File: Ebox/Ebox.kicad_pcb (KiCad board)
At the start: 2 copper layers, 61 x 53.3 mm, 3 parts, among them J1 Screw_Terminal_01x12, J2 Screw_Terminal_01x12

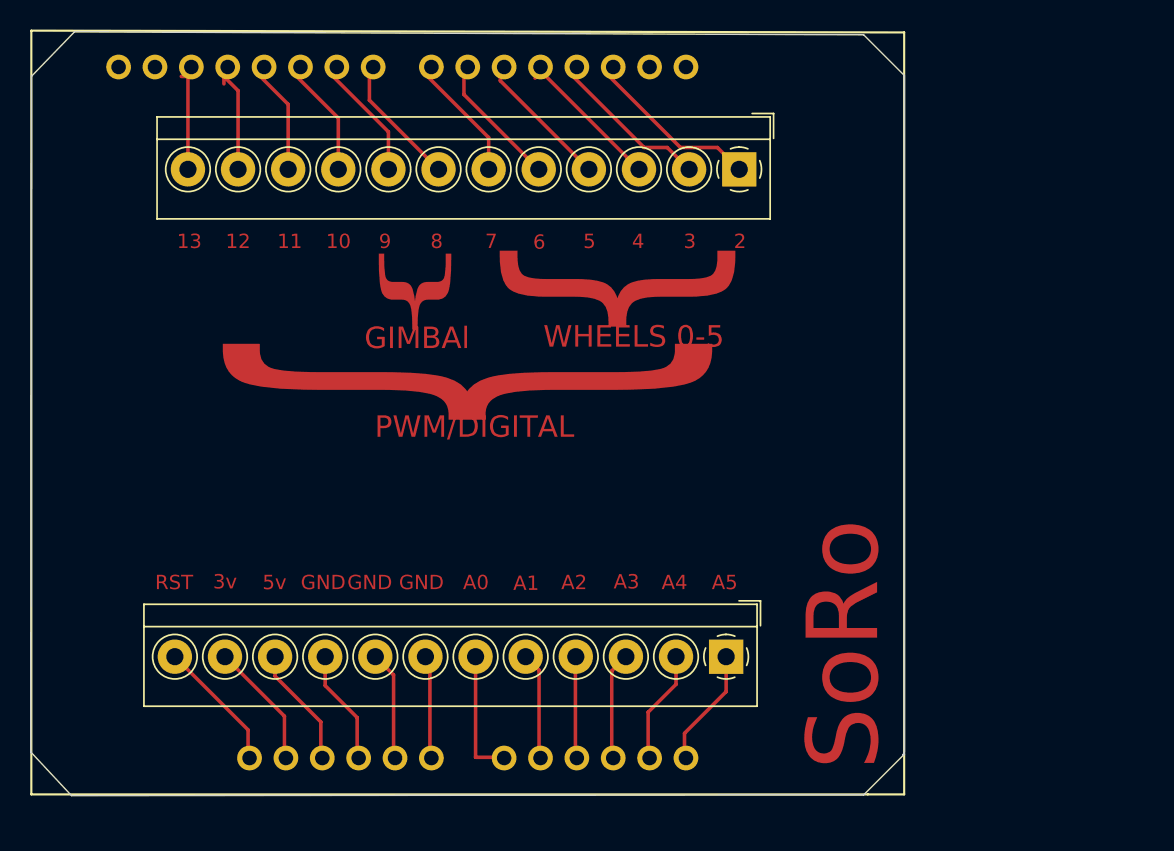
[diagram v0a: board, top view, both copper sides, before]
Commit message: updated Arm arduino code, manual_operate, and PCBs
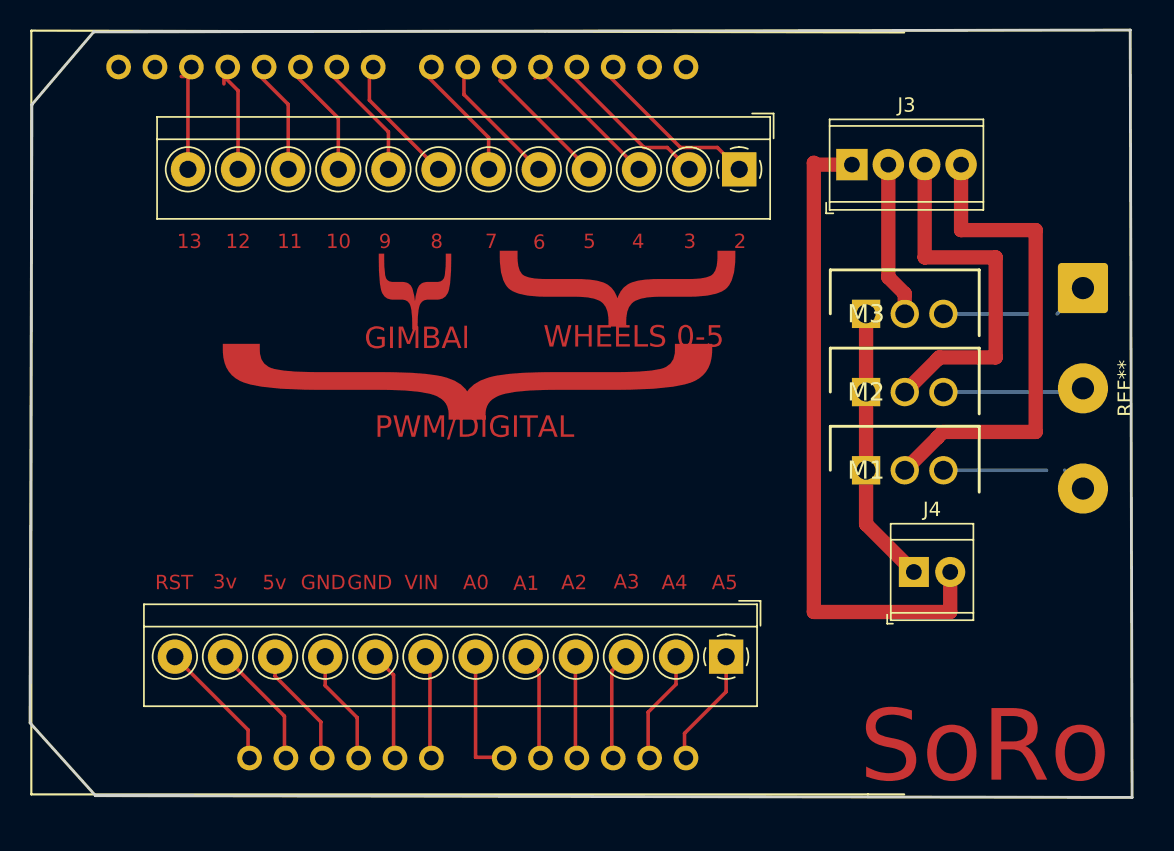
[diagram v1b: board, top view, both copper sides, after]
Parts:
- added J3: Screw_Terminal_01x04, TerminalBlock_Phoenix:TerminalBlock_Phoenix_MPT-0,5-4-2.54_1x04_P2.54mm_Horizontal, F.Cu at (134.1, 63.9)
- added J4: Screw_Terminal_01x02, TerminalBlock_TE-Connectivity:TerminalBlock_TE_282834-2_1x02_P2.54mm_Horizontal, F.Cu at (138.4, 92.3)
- added M1: MNMOS, IRF520:TO270P460X1020X2008-3P, F.Cu at (135.1, 85.2)
- added M2: MNMOS, IRF520:TO270P460X1020X2008-3P, F.Cu at (135.1, 79.8)
- added M3: MNMOS, IRF520:TO270P460X1020X2008-3P, F.Cu at (135.1, 74.3)
- added REF**: SolderWire-0.75sqmm_1x03_P7mm_D1.25mm_OD3.5mm, Connector_Wire:SolderWire-0.75sqmm_1x03_P7mm_D1.25mm_OD3.5mm, F.Cu at (150.2, 72.5)
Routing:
- net Net-(J3-Pad1): track 0.00 -> 46.4 mm
- net Net-(J3-Pad4): track 0.00 -> 34.1 mm
- net Net-(J3-Pad3): track 0.00 -> 25.8 mm
- net Net-(J4-Pad1): track 0.00 -> 19.6 mm
- net Net-(J3-Pad2): track 0.00 -> 10.9 mm
- net Net-(XA1-PadD28): track 0.00 -> 10.2 mm
- net Net-(XA1-PadD26): track 0.00 -> 9.22 mm
- net Net-(XA1-PadD27): track 0.00 -> 8.58 mm
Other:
- board size 61 x 53.3 mm -> 77 x 53.6 mm
- board text added: "VIN"
